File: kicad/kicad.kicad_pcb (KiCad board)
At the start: 2 copper layers, 19.1 x 25.4 mm, 13 parts, among them J1 USB_A_MALE, U1 MCP1702, U2 MCP6021

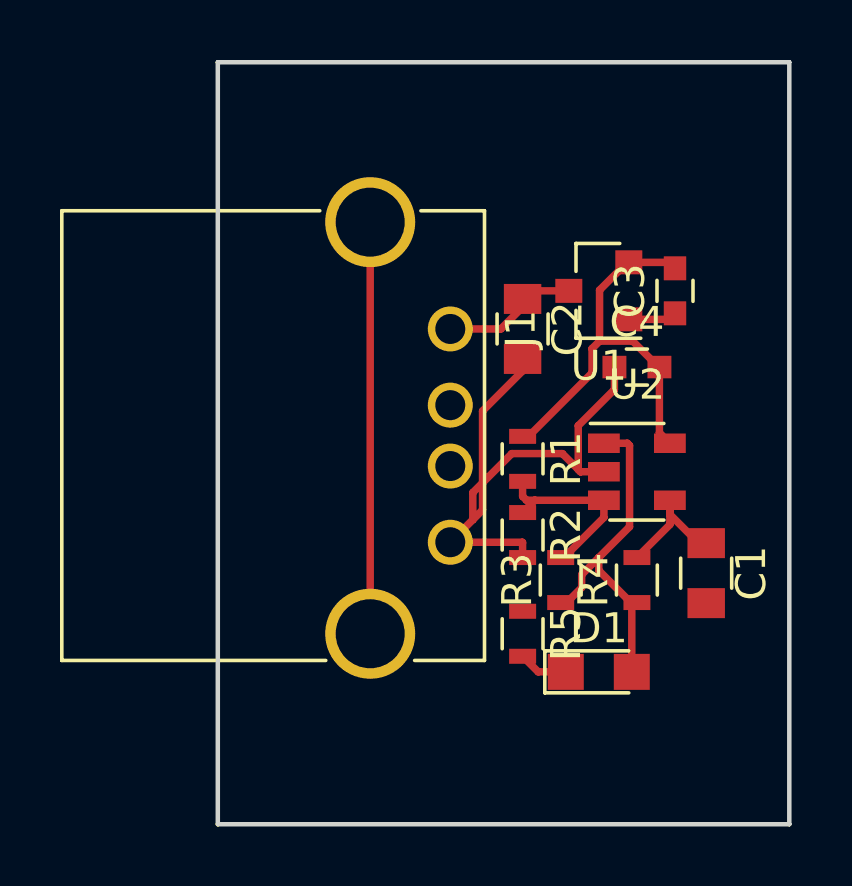
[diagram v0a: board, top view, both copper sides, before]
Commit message: Layout stuff?
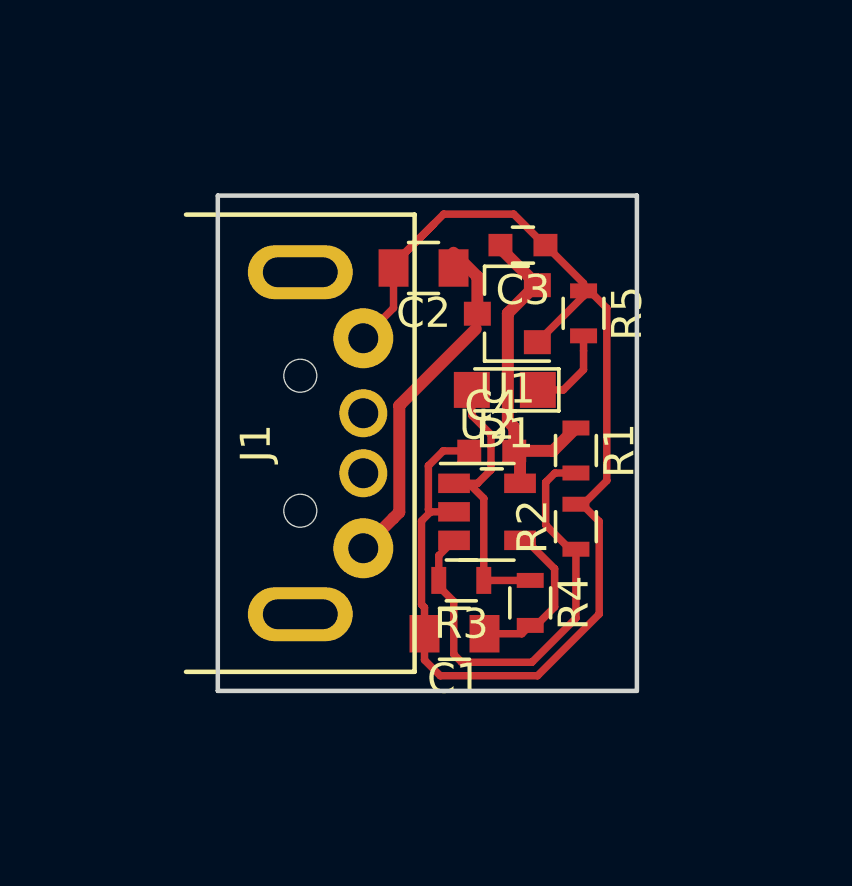
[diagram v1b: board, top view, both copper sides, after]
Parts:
- J1: footprint Connectors:USB_A -> usb_male:USB_A_male
- moved R5 10.9 mm to (151.9, 84.6)
- moved D1 9.91 mm to (149.3, 87.1), turned to 180 degrees
- moved J1 8.64 mm to (139.7, 88.9)
- moved C1 8.63 mm to (147.6, 95.2), turned to 180 degrees
- moved C4 5.59 mm to (148.8, 89.2)
- moved C3 5.29 mm to (149.9, 82.3), turned to 180 degrees
- moved U2 5.17 mm to (148.7, 91.2)
- moved C2 3.88 mm to (146.6, 83.1), turned to 180 degrees
- moved R4 3.64 mm to (150.1, 94.2), turned to 270 degrees
- moved R3 3.31 mm to (147.8, 93.5), turned to 180 degrees
- moved U1 3.14 mm to (149.4, 84.6)
- moved R1 1.80 mm to (151.6, 89.1)
- moved R2 1.80 mm to (151.6, 91.7), turned to 90 degrees
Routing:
- net GND: track 22.3 -> 43.5 mm
- net Net-(J1-Pad5): track 13.7 -> 0.00 mm
- net Net-(R1-Pad2): track 6.41 -> 15.2 mm
- net Net-(C2-Pad1): track 4.49 -> 11.3 mm
- net +3V3: track 14.1 -> 11.4 mm
- net /blink: track 11.7 -> 9.83 mm
- net Net-(D1-Pad1): track 1.66 -> 2.93 mm
- net Net-(C1-Pad1): track 4.55 -> 5.53 mm
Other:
- board size 19.1 x 25.4 mm -> 14 x 16.5 mm
- net class Power added: clearance 0.2, trace_width 0.4, via_dia 0.6, via_drill 0.4

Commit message: Finished layout
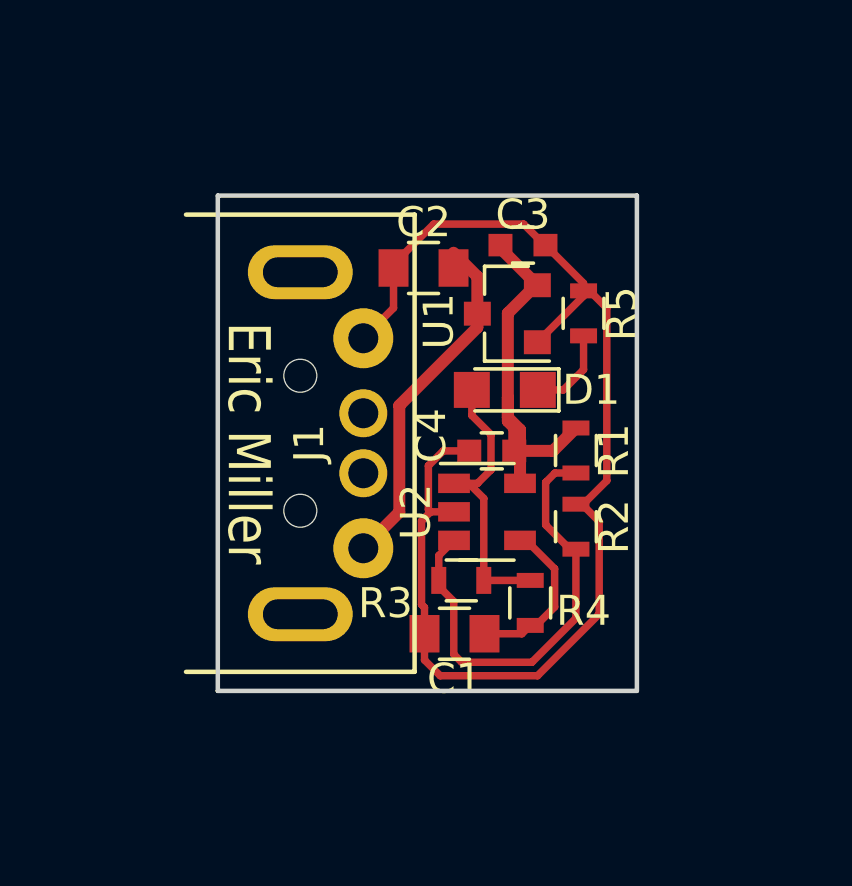
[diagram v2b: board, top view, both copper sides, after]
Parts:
- C1: value 10u -> 10 uf
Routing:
- net +3V3: track 11.4 -> 14.5 mm
- net GND: track 43.5 -> 41.3 mm
- net Net-(C2-Pad1): track 11.3 -> 11.8 mm
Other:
- rule trace_min: 0.2 -> 0.1524
- board text added: "Eric Miller"

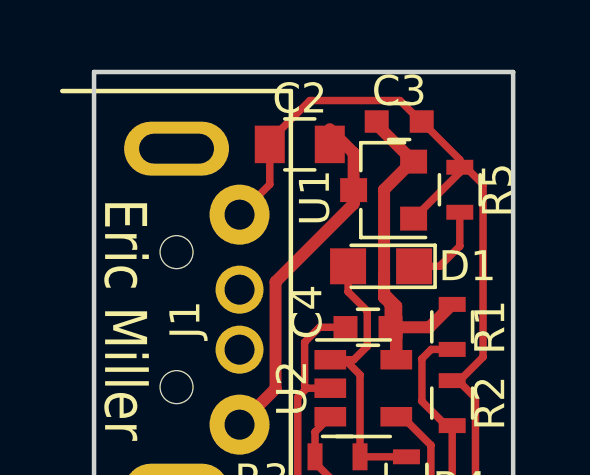
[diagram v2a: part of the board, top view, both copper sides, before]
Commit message: Exported sensitivity and schematic
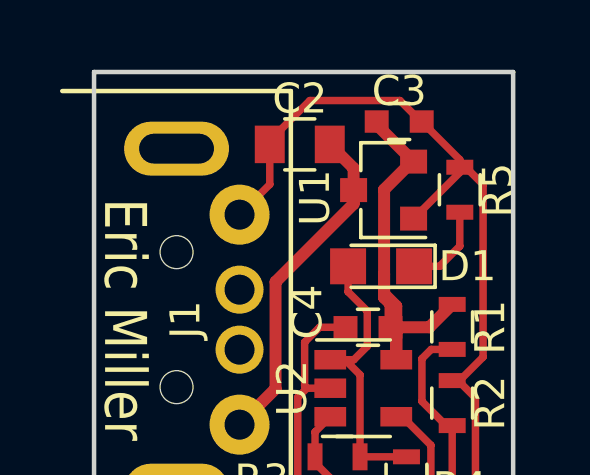
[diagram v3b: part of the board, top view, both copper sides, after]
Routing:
- net Net-(C2-Pad1): track 11.8 -> 11.3 mm
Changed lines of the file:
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@@
     (area 139.624999 80.569999 153.745001 97.230001)
     (thickness 1.6)
-    (drawings 5)
+    (drawings 7)
     (tracks 87)
     (zones 0)
@@
     )
   )
+  (dimension 15.24 (width 0.3) (layer F.SilkS)
+    (gr_text "15.240 mm" (at 128.952 88.9 90) (layer F.SilkS)
+      (effects (font (size 1.5 1.5) (thickness 0.3)))
+    )
+    (feature1 (pts (xy 134.366 81.28) (xy 127.602 81.28)))
+    (feature2 (pts (xy 134.366 96.52) (xy 127.602 96.52)))
+    (crossbar (pts (xy 130.302 96.52) (xy 130.302 81.28)))
+    (arrow1a (pts (xy 130.302 81.28) (xy 130.888421 82.406504)))
+    (arrow1b (pts (xy 130.302 81.28) (xy 129.715579 82.406504)))
+    (arrow2a (pts (xy 130.302 96.52) (xy 130.888421 95.393496)))
+    (arrow2b (pts (xy 130.302 96.52) (xy 129.715579 95.393496)))
+  )
+  (dimension 6.604 (width 0.3) (layer F.SilkS)
+    (gr_text "6.604 mm" (at 143.002 102.442) (layer F.SilkS)
+      (effects (font (size 1.5 1.5) (thickness 0.3)))
+    )
+    (feature1 (pts (xy 139.7 99.822) (xy 139.7 103.792)))
+    (feature2 (pts (xy 146.304 99.822) (xy 146.304 103.792)))
+    (crossbar (pts (xy 146.304 101.092) (xy 139.7 101.092)))
+    (arrow1a (pts (xy 139.7 101.092) (xy 140.826504 100.505579)))
+    (arrow1b (pts (xy 139.7 101.092) (xy 140.826504 101.678421)))
+    (arrow2a (pts (xy 146.304 101.092) (xy 145.177496 100.505579)))
+    (arrow2b (pts (xy 146.304 101.092) (xy 145.177496 101.678421)))
+  )
   (gr_text "Eric Miller" (at 140.716 88.9 270) (layer F.SilkS)
     (effects (font (size 1.4 1.2) (thickness 0.25)))
@@
   (segment (start 150.927999 93.084999) (end 149.979 92.136) (width 0.25) (layer F.Cu) (net 2) (status 20))
   (segment (start 149.979 92.136) (end 149.774 92.136) (width 0.25) (layer F.Cu) (net 2) (status 30))
+  (segment (start 148.352 84.582) (end 148.352 83.852) (width 0.4) (layer F.Cu) (net 3) (status 10))
+  (segment (start 148.352 83.852) (end 147.558 83.058) (width 0.4) (layer F.Cu) (net 3) (status 20))
   (segment (start 148.352 84.582) (end 148.352 85.04) (width 0.4) (layer F.Cu) (net 3) (status 10))
   (segment (start 148.352 85.04) (end 145.750001 87.641999) (width 0.4) (layer F.Cu) (net 3))
@@
   (segment (start 145.750001 91.199999) (end 144.55 92.4) (width 0.4) (layer F.Cu) (net 3) (status 20))
   (segment (start 148.352 84.582) (end 148.302 84.582) (width 0.4) (layer F.Cu) (net 3) (status 30))
-  (segment (start 148.352 84.582) (end 148.352 83.344) (width 0.4) (layer F.Cu) (net 3) (status 10))
-  (segment (start 148.352 83.344) (end 147.558 82.55) (width 0.4) (layer F.Cu) (net 3) (status 20))
   (segment (start 149.367999 84.566001) (end 149.367999 87.376) (width 0.4) (layer F.Cu) (net 4))
   (segment (start 149.367999 87.376) (end 149.367999 88.164999) (width 0.4) (layer F.Cu) (net 4))
-  (segment (start 149.774 90.236) (end 149.774 88.448002) (width 0.4) (layer F.Cu) (net 4))
+  (segment (start 149.774 90.236) (end 149.774 88.448002) (width 0.4) (layer F.Cu) (net 4) (status 10))
   (segment (start 149.774 88.448002) (end 149.367999 88.042001) (width 0.4) (layer F.Cu) (net 4))
   (segment (start 149.367999 88.042001) (end 149.367999 87.376) (width 0.4) (layer F.Cu) (net 4))
